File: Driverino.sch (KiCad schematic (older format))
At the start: 54 parts, among them P1 ICSP/SPI, P2 USB, P3 RS232, P4 PWR_IN, P5 HALL, P6 MOT, U1 MCT8316Z, U2 ATmega32U4, U3 ADM3101EACPZ-250R7, Y1 16MHz

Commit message: Defined schematics hierarchy
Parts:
- removed C1: 150uF, symbol device:CP1
- removed C10, C8, C9: 100nF 16V, Capacitor_SMD:C_0603_1608Metric, symbol device:C
- removed C11, C14: 1uF 16V 10%, Capacitor_SMD:C_0603_1608Metric, symbol device:C
- removed C12, C15, C17, C20, C21: 0.1uF 16V 10%, Capacitor_SMD:C_0603_1608Metric, symbol device:C
- removed C13: 100nF 6.3V, Capacitor_SMD:C_0603_1608Metric, symbol device:C
- removed C16: 100nF 16V 10%, Capacitor_SMD:C_0603_1608Metric, symbol device:C
- removed C18, C19: 18pF, Capacitor_SMD:C_0402_1005Metric, symbol device:C
- removed C2: 10uF 50V, Capacitor_SMD:C_0603_1608Metric, symbol device:C
- removed C3: 1uF 16V, Capacitor_SMD:C_0603_1608Metric, symbol device:C
- removed C4: 100nF 100V, Capacitor_SMD:C_0603_1608Metric, symbol device:C
- removed C5: 10nF 50V, Capacitor_SMD:C_0603_1608Metric, symbol device:C
- removed C6: 1uF 6.3V, Capacitor_SMD:C_0603_1608Metric, symbol device:C
- removed C7: 22uF, symbol device:C
- removed D1: YEL, LED_SMD:LED_0603_1608Metric, symbol device:LED
- removed D2: VZ=3V, Diode_SMD:D_SOD-523, symbol device:ZENERsmall
- removed D3: GREEN, LED_SMD:LED_0603_1608Metric, symbol device:LED
- removed L1: 47uH, symbol device:INDUCTOR_SMALL
- removed P1: ICSP/SPI, Connector_Molex:Molex_PicoBlade_53047-0710_1x07_P1.25mm_Vertical, symbol conn:CONN_7
- removed P2: USB, Connector_Molex:Molex_PicoBlade_53047-0410_1x04_P1.25mm_Vertical, symbol conn:CONN_4
- removed P3: RS232, Connector_Molex:Molex_PicoBlade_53047-0310_1x03_P1.25mm_Vertical, symbol conn:CONN_3
- removed P4: PWR_IN, Connector_Molex:Molex_PicoBlade_53047-0210_1x02_P1.25mm_Vertical, symbol conn:CONN_2
- removed P5: HALL, Connector_Molex:Molex_PicoBlade_53047-0810_1x03_P1.25mm_Vertical, symbol conn:CONN_8
- removed P6: MOT, Connector_Molex:Molex_PicoBlade_53047-0310_1x03_P1.25mm_Vertical, symbol conn:CONN_3
- removed R1, R2: 5.1k, Resistor_SMD:R_0402_1005Metric, symbol device:R
- removed R10, R14, R15, R17, R19, R9: 0R, Resistor_SMD:R_0603_1608Metric, symbol device:R
- removed R11, R12: 22R, Resistor_SMD:R_0603_1608Metric, symbol device:R
- removed R13, R16, R18, R5: 10k 1% 1/16W, Resistor_SMD:R_0402_1005Metric, symbol device:R
- removed R3, R6, R7: R DNM, Resistor_SMD:R_0603_1608Metric, symbol device:R
- removed R4, R8: 332R, Resistor_SMD:R_0603_1608Metric, symbol device:R
- removed U1: MCT8316Z, symbol texas2:MCT8316Z
- removed U2: ATmega32U4, Package_QFP:TQFP-44_10x10mm_P0.8mm, symbol V2-30A110-A-symbols:ATmega32U4
- removed U3: ADM3101EACPZ-250R7, CP_12_1, symbol ad:ADM3101EACPZ-250R7
- removed Y1: 16MHz, Crystal:Crystal_SMD_2520-4Pin_2.5x2.0mm, symbol device:CRYSTAL
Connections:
- net labels removed: A0, A1, A2, A3, A4, A5, BRAKE, CS1, CS2, D+, D-, D10, D11, D12, D13, D4, D5, D6, D7, D8, D9, DRVOFF, FAULT, FB, FGOUT, GND, GNDPWR, GND_BK, HAN, HAP, HBN, HBP, HCN, HCP, HT, ILIM, INT, MISO, MOSI, PWM, RAW, RESET, RXI, RX_232, SCK, SCL, SDA, SLEEP, SW, TXO, TX_232, U, UVCC, V, VCC, VDD, W
- wire segments 295 -> 10
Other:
- note removed: "TODO: micro leds? pwr leds? fault led?"

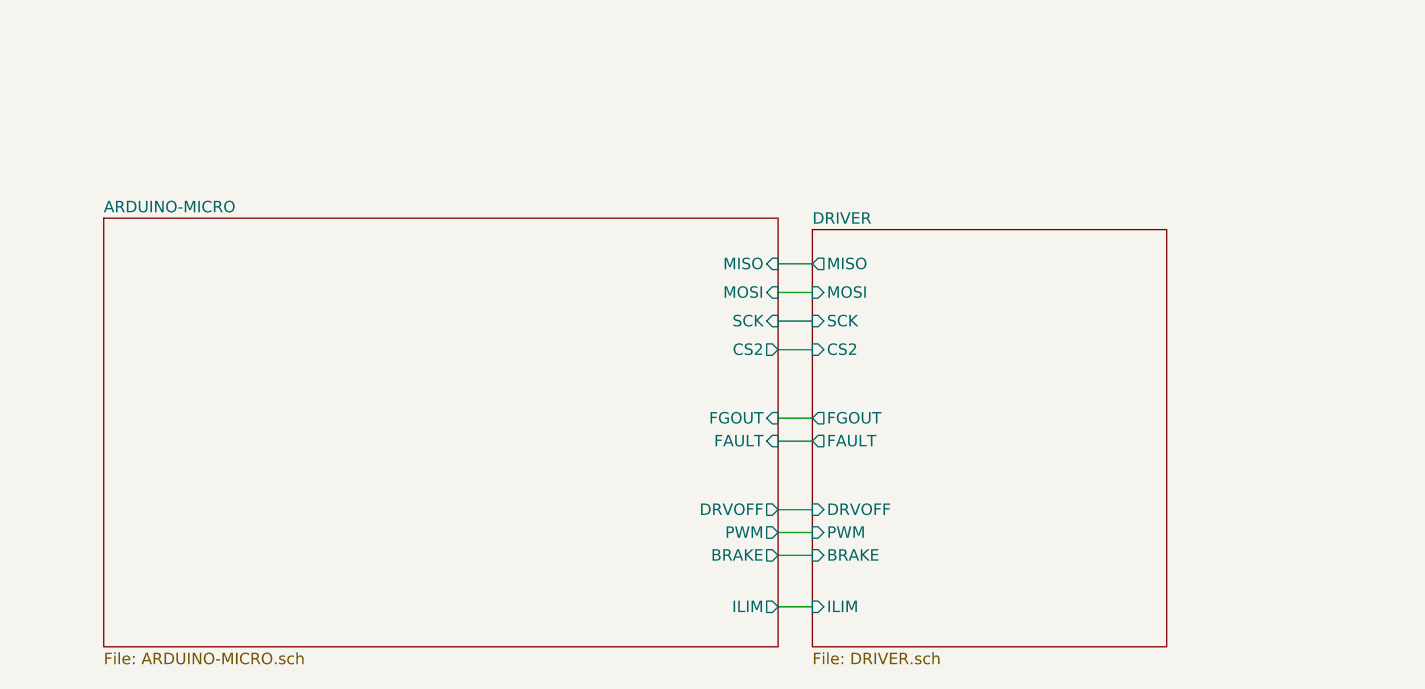
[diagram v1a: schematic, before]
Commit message: Update
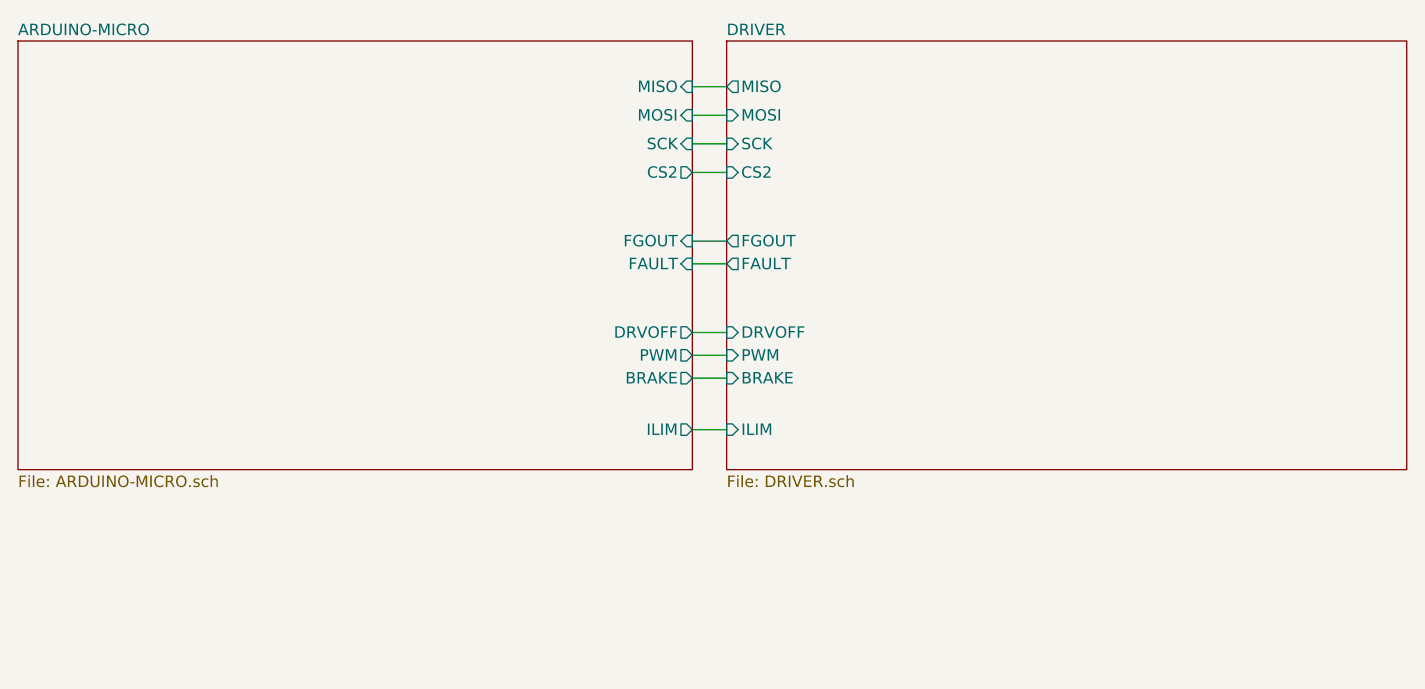
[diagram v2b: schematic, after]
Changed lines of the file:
@@
 $EndDescr
 $Sheet
-S 6300 3300 1550 1825
+S 2825 2475 2950 1875
+U 614792E0
+F0 "ARDUINO-MICRO" 50
+F1 "ARDUINO-MICRO.sch" 50
+F2 "MISO" I R 5775 2675 50
+F3 "SCK" I R 5775 2925 50
+F4 "MOSI" I R 5775 2800 50
+F5 "ILIM" O R 5775 4175 50
+F6 "FGOUT" I R 5775 3350 50
+F7 "FAULT" I R 5775 3450 50
+F8 "DRVOFF" O R 5775 3750 50
+F9 "PWM" O R 5775 3850 50
+F10 "BRAKE" O R 5775 3950 50
+F11 "CS2" O R 5775 3050 50
+$EndSheet
+Wire Wire Line
+	5775 2675 5925 2675
+Wire Wire Line
+	5775 2800 5925 2800
+Wire Wire Line
+	5775 2925 5925 2925
+Wire Wire Line
+	5775 4175 5925 4175
+Wire Wire Line
+	5775 3350 5925 3350
+Wire Wire Line
+	5925 3450 5775 3450
+Wire Wire Line
+	5775 3750 5925 3750
+Wire Wire Line
+	5775 3850 5925 3850
+Wire Wire Line
+	5775 3950 5925 3950
+Wire Wire Line
+	5775 3050 5925 3050
+$Sheet
+S 5925 2475 2975 1875
 U 613CDDB7
 F0 "DRIVER" 50
 F1 "DRIVER.sch" 50
-F2 "FGOUT" O L 6300 4125 50
-F3 "PWM" I L 6300 4625 50
-F4 "BRAKE" I L 6300 4725 50
-F5 "ILIM" I L 6300 4950 50
-F6 "CS2" I L 6300 3825 50
-F7 "SCK" I L 6300 3700 50
-F8 "MOSI" I L 6300 3575 50
-F9 "MISO" O L 6300 3450 50
-F10 "DRVOFF" I L 6300 4525 50
-F11 "FAULT" O L 6300 4225 50
+F2 "FGOUT" O L 5925 3350 50
+F3 "PWM" I L 5925 3850 50
+F4 "BRAKE" I L 5925 3950 50
+F5 "ILIM" I L 5925 4175 50
+F6 "CS2" I L 5925 3050 50
+F7 "SCK" I L 5925 2925 50
+F8 "MOSI" I L 5925 2800 50
+F9 "MISO" O L 5925 2675 50
+F10 "DRVOFF" I L 5925 3750 50
+F11 "FAULT" O L 5925 3450 50
 $EndSheet
-$Sheet
-S 3200 3250 2950 1875
-U 614792E0
-F0 "ARDUINO-MICRO" 50
-F1 "ARDUINO-MICRO.sch" 50
-F2 "MISO" I R 6150 3450 50
-F3 "SCK" I R 6150 3700 50
-F4 "MOSI" I R 6150 3575 50
-F5 "ILIM" O R 6150 4950 50
-F6 "FGOUT" I R 6150 4125 50
-F7 "FAULT" I R 6150 4225 50
-F8 "DRVOFF" O R 6150 4525 50
-F9 "PWM" O R 6150 4625 50
-F10 "BRAKE" O R 6150 4725 50
-F11 "CS2" O R 6150 3825 50
-$EndSheet
-Wire Wire Line
-	6150 3450 6300 3450
-Wire Wire Line
-	6150 3575 6300 3575
-Wire Wire Line
-	6150 3700 6300 3700
-Wire Wire Line
-	6150 4950 6300 4950
-Wire Wire Line
-	6150 4125 6300 4125
-Wire Wire Line
-	6300 4225 6150 4225
-Wire Wire Line
-	6150 4525 6300 4525
-Wire Wire Line
-	6150 4625 6300 4625
-Wire Wire Line
-	6150 4725 6300 4725
-Wire Wire Line
-	6150 3825 6300 3825
 $EndSCHEMATC
